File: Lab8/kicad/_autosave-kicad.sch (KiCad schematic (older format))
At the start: 17 parts, among them J4 TI_BOOSTER_40_J4

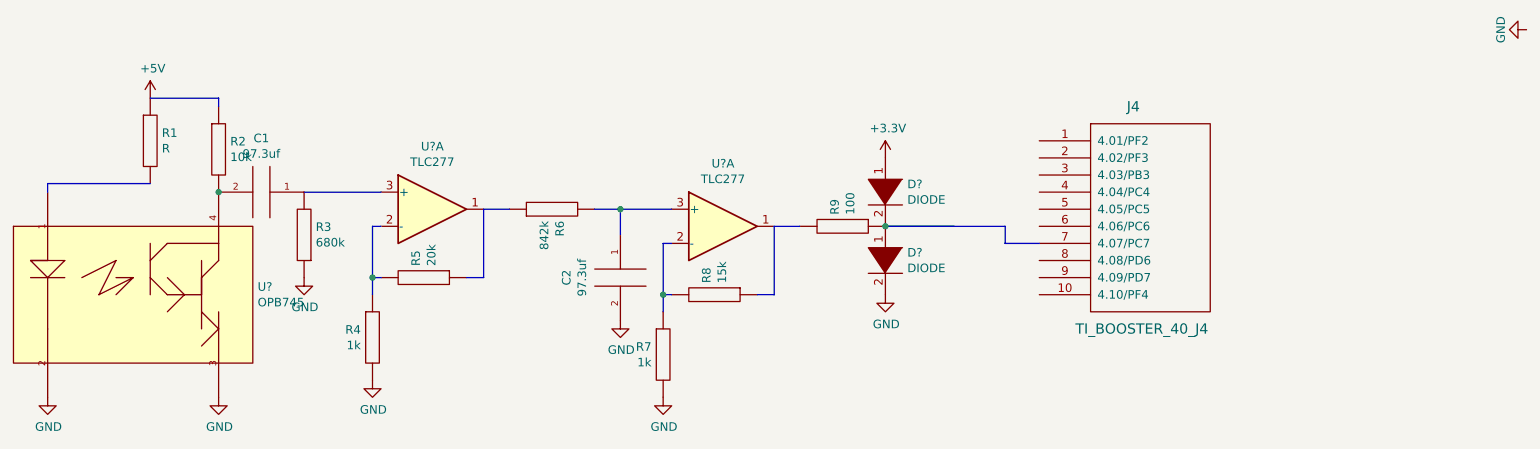
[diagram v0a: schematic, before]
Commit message: nearly done w/ lab08
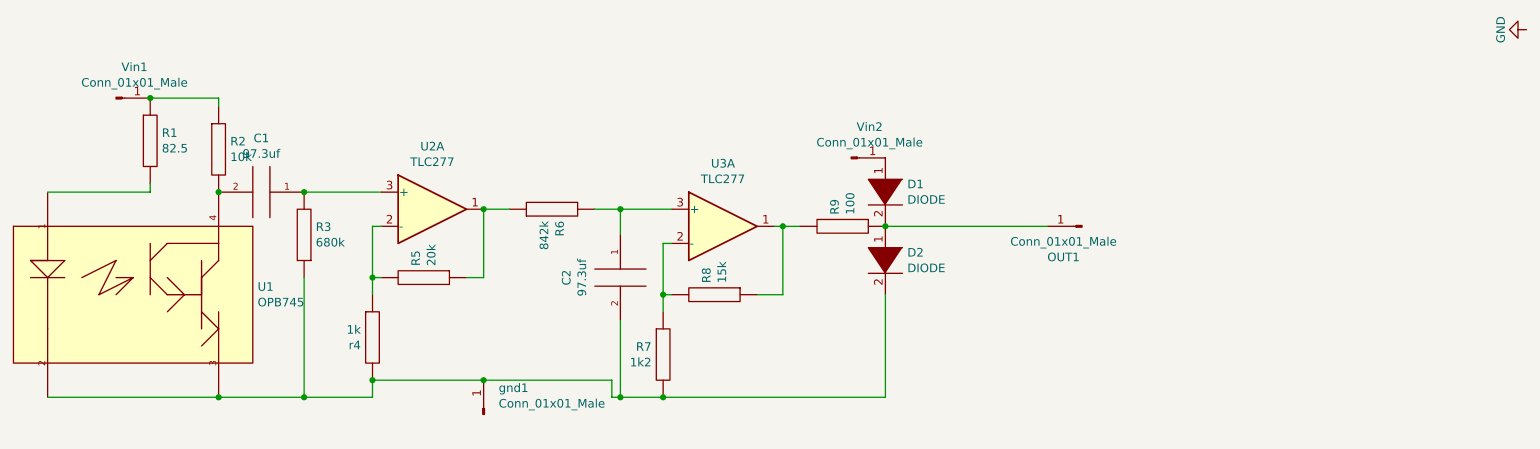
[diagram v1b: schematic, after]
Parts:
- removed J4: TI_BOOSTER_40_J4, Connector_PinHeader_2.54mm:PinHeader_1x10_P2.54mm_Vertical, symbol boosterpack:Ti_Booster_40_J4
- added OUT1, gnd1: Conn_01x01_Male, Connector_PinHeader_2.54mm:PinHeader_1x07_P2.54mm_Vertical_SMD_Pin1Left, symbol Connector:Conn_01x01_Male
- added Vin1, Vin2: Conn_01x01_Male, Connector_PinHeader_2.54mm:PinHeader_1x08_P2.54mm_Vertical_SMD_Pin1Left, symbol Connector:Conn_01x01_Male
- 1k2: renamed from 1k; footprint (none) -> Resistor_SMD:R_0201_0603Metric
- C1: footprint (none) -> Capacitor_SMD:CP_Elec_3x5.4
- C2: footprint (none) -> Capacitor_SMD:CP_Elec_4x3
- D1, D2: renamed from D?; footprint (none) -> Diode_SMD:D_0201_0603Metric
- R1: value R -> 82.5; footprint (none) -> Resistor_SMD:R_0201_0603Metric
- R2, R3, R5, R6, R8, R9: footprint (none) -> Resistor_SMD:R_0201_0603Metric
- U1: renamed from U?; footprint TT_Electronics-OPB745-* -> Connector_PinSocket_2.54mm:PinSocket_1x08_P2.54mm_Vertical
- U2, U3: renamed from U?; footprint (none) -> TLC277CP:DIP794W45P254L959H508Q8
- r4: renamed from 1k; value R4 -> 1k; footprint (none) -> Resistor_SMD:R_0201_0603Metric
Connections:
- net +5V is gone; now on an unnamed net: R1.1
- net GND: no longer 1k2.2, C2.2, D2.2 (A), R3.1, U1.2 (Cathode), U1.3 (Emitter), r4.2
- net at R1.2: now also U1.1 (Anode)
- net at R2.1: now also Vin1.1 (Pin_1)
- net at C1.1, R3.2: now also U2.3 (+)
- net at U2.1: now also R5.1, R6.1
- net at U2.2 (-): now also R5.2, r4.1
- net at R6.2: now also C2.1, U3.3 (+)
- net at U3.1: now also R8.1, R9.2
- net at U3.2 (-): now also 1k2.1, R8.2
- net at D1.2 (A), D2.1 (K), R9.1: now also OUT1.1 (Pin_1)
- net +3V3: no longer names the net of D1.1 (K)
- net +3V3: now also Vin2.1 (Pin_1)
- new net: 1k2.2, C2.2, D2.2 (A), R3.1, U1.2 (Cathode), U1.3 (Emitter), gnd1.1 (Pin_1), r4.2
